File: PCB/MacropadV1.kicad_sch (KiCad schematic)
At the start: 17 parts, among them J1 Conn_01x04, SW1 SW_Push, SW10 RotaryEncoder_Switch, SW2 SW_Push, SW3 SW_Push, SW4 SW_Push, SW5 SW_Push, SW6 SW_Push, U1 MOUDLE-SEEEDUINO-XIAO

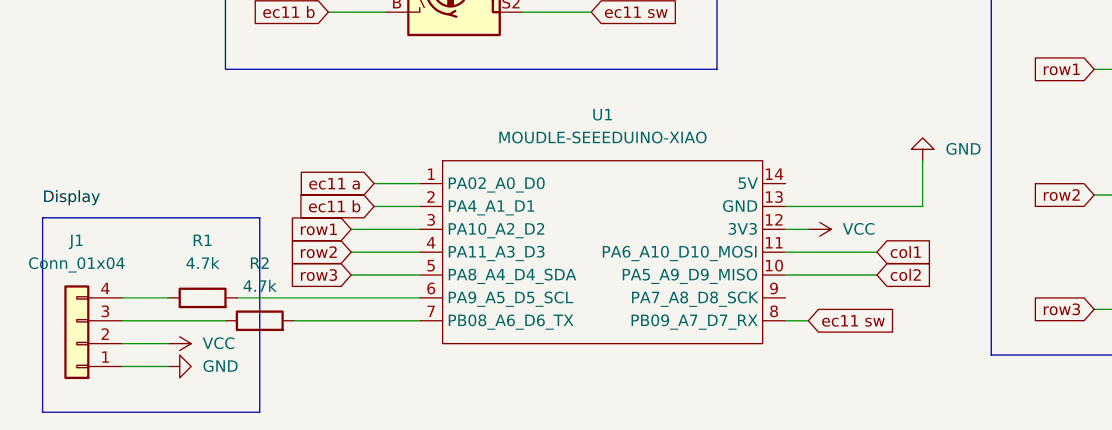
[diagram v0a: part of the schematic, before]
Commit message: added bom file
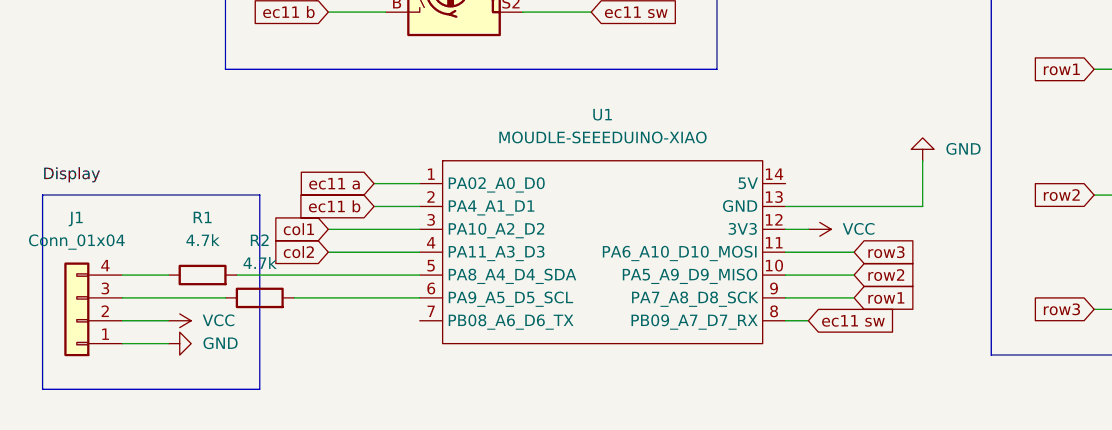
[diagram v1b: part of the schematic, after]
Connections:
- net col1: now also U1.3 (PA10_A2_D2); no longer U1.11 (PA6_A10_D10_MOSI)
- net col2: now also U1.4 (PA11_A3_D3); no longer U1.10 (PA5_A9_D9_MISO)
- net row1: now also U1.9 (PA7_A8_D8_SCK); no longer U1.3 (PA10_A2_D2)
- net row2: now also U1.10 (PA5_A9_D9_MISO); no longer U1.4 (PA11_A3_D3)
- net row3: now also U1.11 (PA6_A10_D10_MOSI); no longer U1.5 (PA8_A4_D4_SDA)
- net at R2.2: now also U1.6 (PA9_A5_D5_SCL); no longer U1.7 (PB08_A6_D6_TX)
- net at R1.2: now also U1.5 (PA8_A4_D4_SDA); no longer U1.6 (PA9_A5_D5_SCL)
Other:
- moved on the sheet: J1, R1, R2
